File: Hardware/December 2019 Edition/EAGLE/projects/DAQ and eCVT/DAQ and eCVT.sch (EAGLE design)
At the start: 78 parts, among them J1 10118193-0001LF, J2 TBL004-508-06BE-2GY, J3 TBL004-508-06BE-2GY, J4 TBL004-508-06BE-2GY, J5 TBL004-508-06BE-2GY, J6 TBL004-508-06BE-2GY, J7 TBL004-508-06BE-2GY

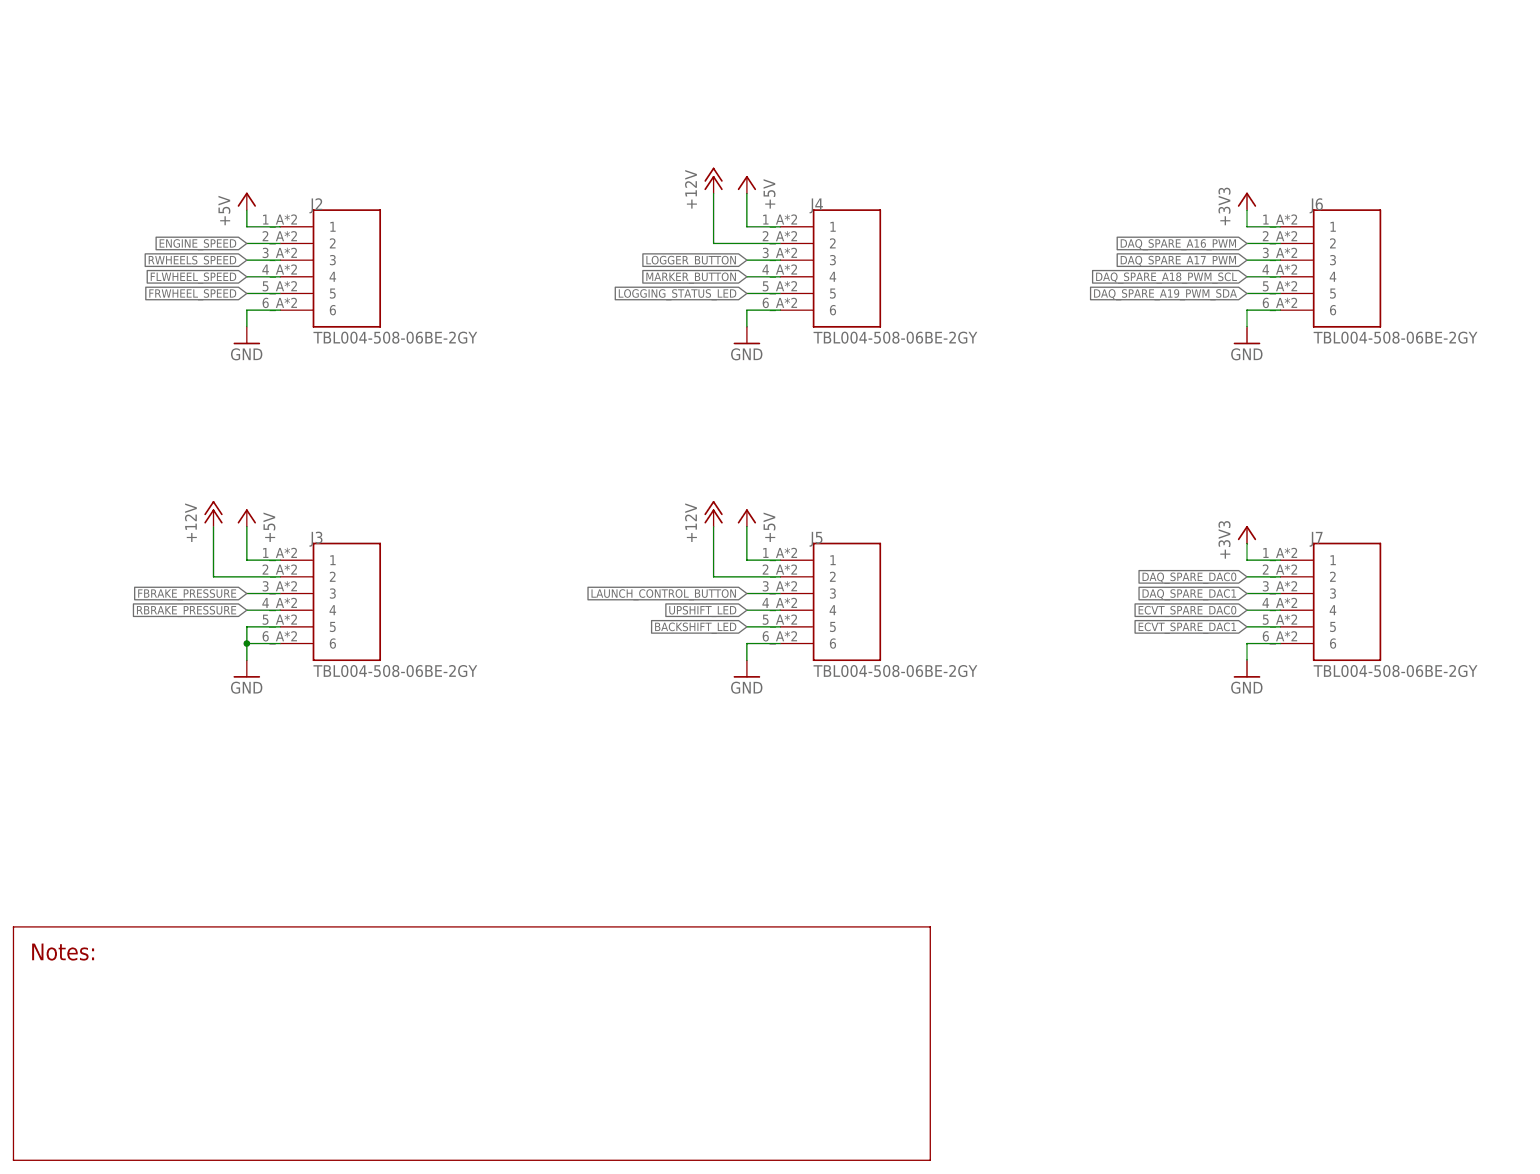
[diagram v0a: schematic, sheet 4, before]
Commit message: Finished schematic!
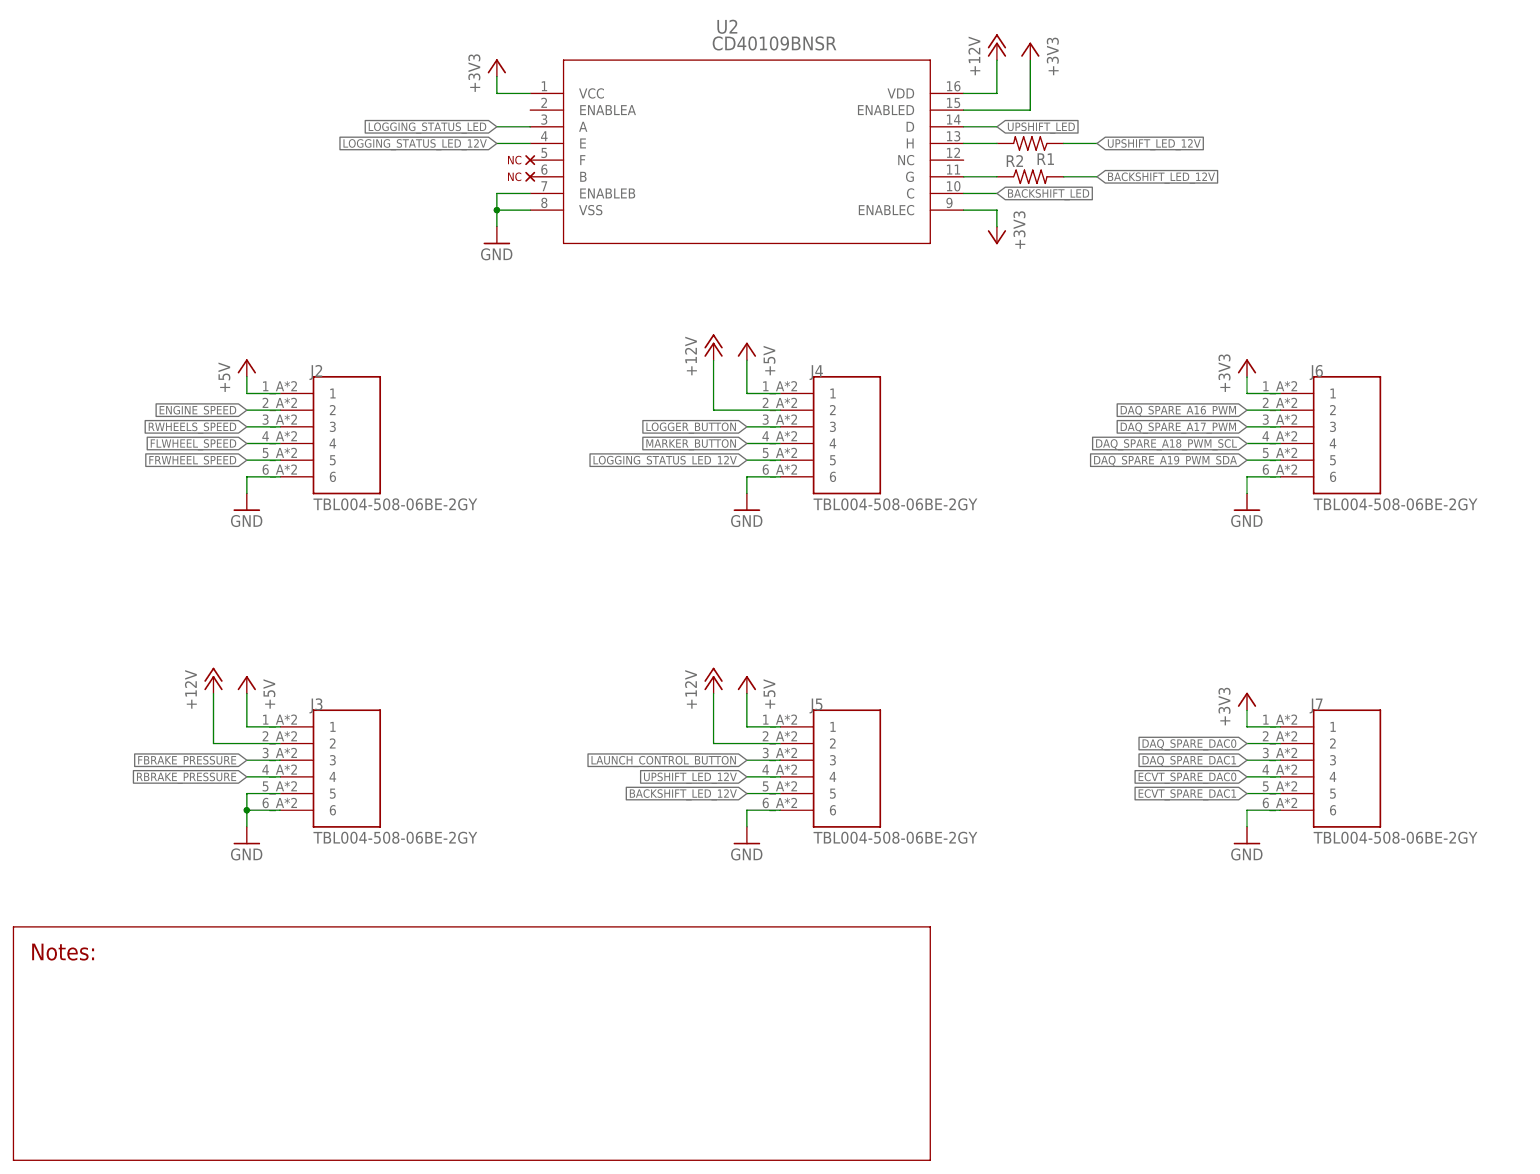
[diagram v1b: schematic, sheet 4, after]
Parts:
- removed CR2: ST26C32ABDR, Quadruple Line Receiver:ST26C32ABDR
- added R1, R2: (no value), rcl:R-US_0204/7
- added U$67, U$68: NC, ME 507:NC
- added U1: AM26LS32ACDR, Quad. Diff. Line Receiver:AM26LS32ACDR
- added U2: CD40109BNSR, Quad. Level Shifter:CD40109BNSR
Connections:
- new net BACKSHIFT_LED_12V: J5.5, R2.2
- new net BACKSHIFT_LED_12V_W/O_RES: R2.1, U2.G
- new net LOGGING_STATUS_LED_12V: J4.5, U2.E
- new net N$58: U$67.D, U2.F
- new net N$60: U$68.D, U2.B
- new net UPSHIFT_LED_12V: J5.4, R1.1
- new net UPSHIFT_LED_12V_W/O_RES: R1.2, U2.H
- net +12V: now also U2.VDD
- net +3V3: now also U2.ENABLEC, U2.ENABLED, U2.VCC
- net +5V: now also U1.G, U1.VCC; no longer CR2.EN, CR2.VCC
- net BACKSHIFT_LED: now also U2.C; no longer J5.5
- net GND: now also U1.!G, U1.GND, U2.ENABLEB, U2.VSS; no longer CR2.!, CR2.GND
- net LOGGING_STATUS_LED: now also U2.A; no longer J4.5
- net P_ENC_A: now also U1.1Y; no longer CR2.AOUT
- net P_ENC_B: now also U1.2Y; no longer CR2.BOUT
- net P_ENC_CHA: now also U1.1A; no longer CR2.AIN2
- net P_ENC_CHA/: now also U1.1B; no longer CR2.AIN1
- net P_ENC_CHB: now also U1.2A; no longer CR2.BIN2
- net P_ENC_CHB/: now also U1.2B; no longer CR2.BIN1
- net S_ENC_A: now also U1.3Y; no longer CR2.COUT
- net S_ENC_B: now also U1.4Y; no longer CR2.DOUT
- net S_ENC_CHA: now also U1.3A; no longer CR2.CIN2
- net S_ENC_CHA/: now also U1.3B; no longer CR2.CIN1
- net S_ENC_CHB: now also U1.4A; no longer CR2.DIN2
- net S_ENC_CHB/: now also U1.4B; no longer CR2.DIN1
- net UPSHIFT_LED: now also U2.D; no longer J5.4
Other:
- moved on the sheet: J2, J3, J4, J5, J6, J7, U$58
